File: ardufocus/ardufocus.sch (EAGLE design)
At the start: 14 parts, among them J5 POWER_JACK, M1 ARDUINO-NANO-3.0, X2 JST-XH-04-PIN-LONG-PAD, X3 JST-XH-04-PIN-LONG-PAD, X4 JST-XH-04-PIN-LONG-PAD, X5 JST-XH-04-PIN-LONG-PAD, X6 JST-XH-02-PIN-LONG-PAD

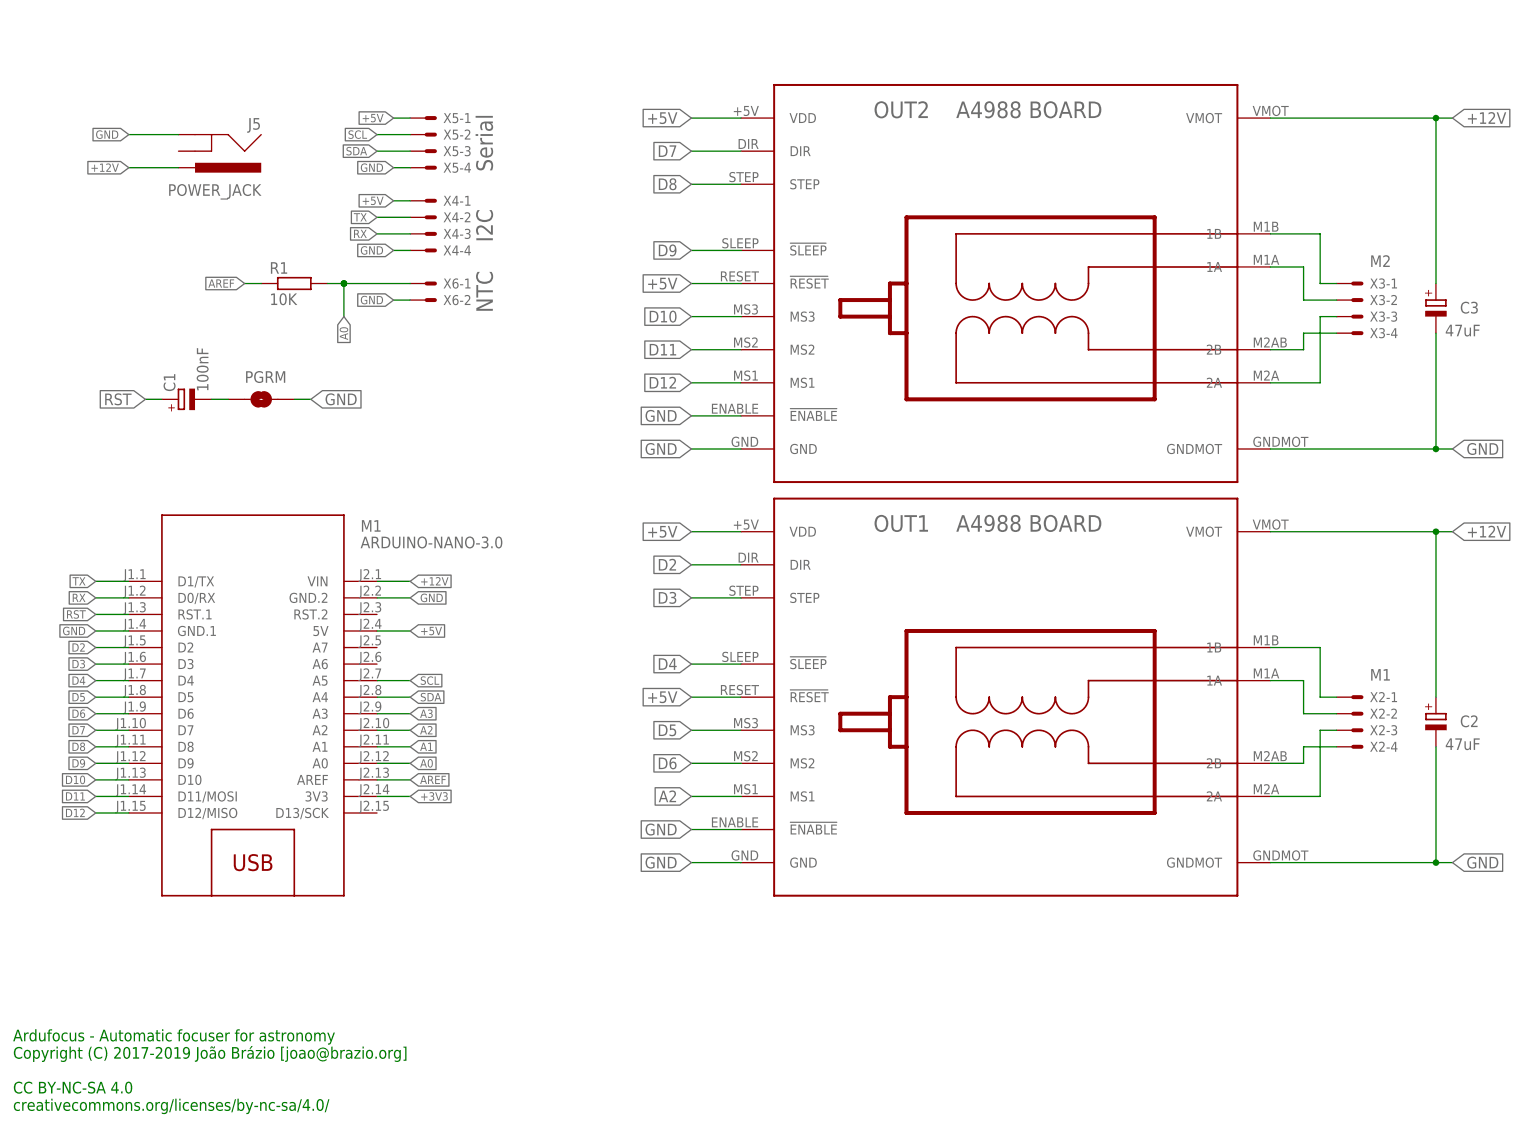
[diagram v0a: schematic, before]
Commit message: New PCB layout
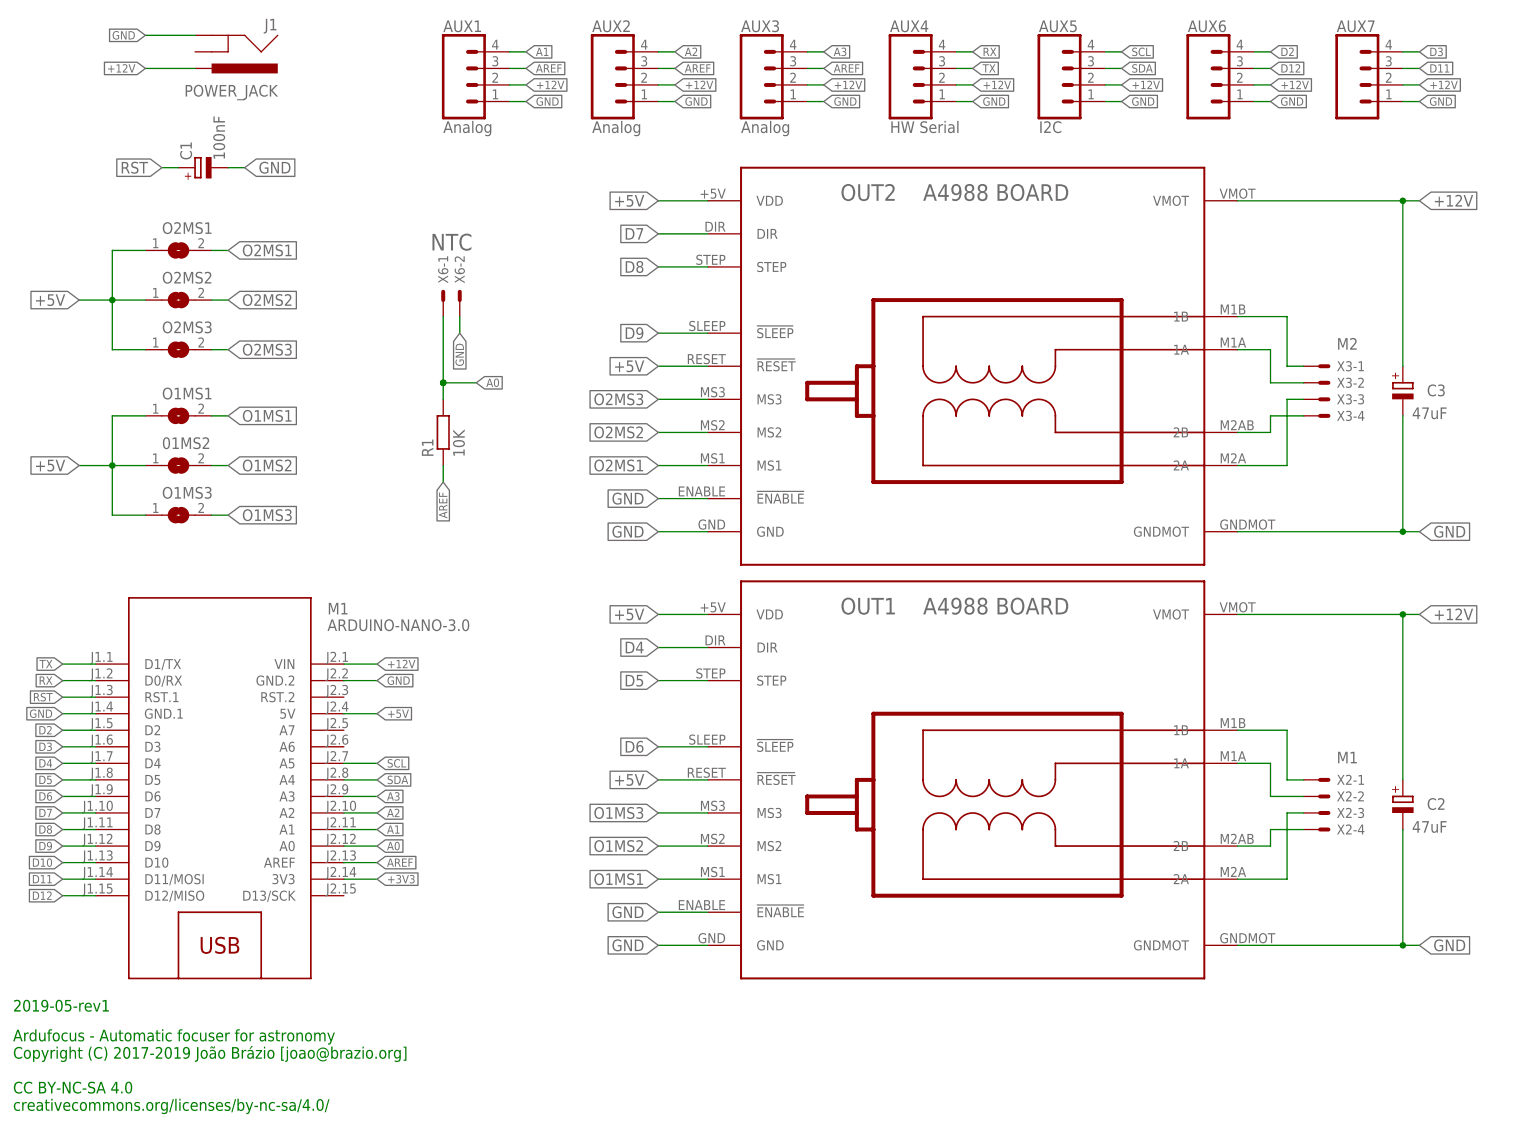
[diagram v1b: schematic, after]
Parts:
- removed J5: POWER_JACK, SparkFun-Connectors:POWER_JACK
- removed PGRM: JUMPER-SMT_2_NO_SILK, SparkFun-Jumpers:JUMPER-SMT_2_NO_SILK
- removed X4, X5: JST-XH-04-PIN-LONG-PAD, jst-xh:JST-XH-04-PIN-LONG-PAD
- added 01MS2, O1MS1, O1MS3, O2MS1, O2MS2, O2MS3: (no value), jumper:SJ
- added AUX1, AUX2, AUX3: Analog, SparkFun-Connectors:CONN_04
- added AUX4: HW Serial, SparkFun-Connectors:CONN_04
- added AUX5: I2C, SparkFun-Connectors:CONN_04
- added AUX6, AUX7: (no value), SparkFun-Connectors:CONN_04
- added J1: POWER_JACK, SparkFun-Connectors:POWER_JACK
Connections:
- removed net N$2: C1.-, PGRM.1
- new net O1MS1: O1MS1.2, OUT1.MS1
- new net O1MS2: 01MS2.2, OUT1.MS2
- new net O1MS3: O1MS3.2, OUT1.MS3
- new net O2MS1: O2MS1.2, OUT2.MS1
- new net O2MS2: O2MS2.2, OUT2.MS2
- new net O2MS3: O2MS3.2, OUT2.MS3
- net +12V: now also AUX1.2, AUX2.2, AUX3.2, AUX4.2, AUX5.2, AUX6.2, AUX7.2, J1.PWR; no longer J5.PWR
- net +5V: now also 01MS2.1, O1MS1.1, O1MS3.1, O2MS1.1, O2MS2.1, O2MS3.1; no longer X4-1.S, X5-1.S
- net A1: now also AUX1.4
- net A2: now also AUX2.4; no longer OUT1.MS1
- net A3: now also AUX3.4
- net AREF: now also AUX1.3, AUX2.3, AUX3.3
- net D10: no longer OUT2.MS3
- net D11: now also AUX7.3; no longer OUT2.MS2
- net D12: now also AUX6.3; no longer OUT2.MS1
- net D2: now also AUX6.4; no longer OUT1.DIR
- net D3: now also AUX7.4; no longer OUT1.STEP
- net D4: now also OUT1.DIR; no longer OUT1.!SLEEP
- net D5: now also OUT1.STEP; no longer OUT1.MS3
- net D6: now also OUT1.!SLEEP; no longer OUT1.MS2
- net GND: now also AUX1.1, AUX2.1, AUX3.1, AUX4.1, AUX5.1, AUX6.1, AUX7.1, C1.-, J1.GND; no longer J5.GND, PGRM.2, X4-4.S, X5-4.S
- net RX: now also AUX4.4; no longer X4-3.S
- net SCL: now also AUX5.4; no longer X5-2.S
- net SDA: now also AUX5.3; no longer X5-3.S
- net TX: now also AUX4.3; no longer X4-2.S
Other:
- note added: "2019-05-rev1"
- note removed: "I2C"
- note removed: "Serial"
- moved on the sheet: C1, C2, C3, M1, OUT1, OUT2, R1, X2-1, X2-2, X2-3, X2-4, X3-1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

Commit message: Revert "New PCB layout"
This reverts commit abb039d9954214917f7d505cd5213ebb6519a360.
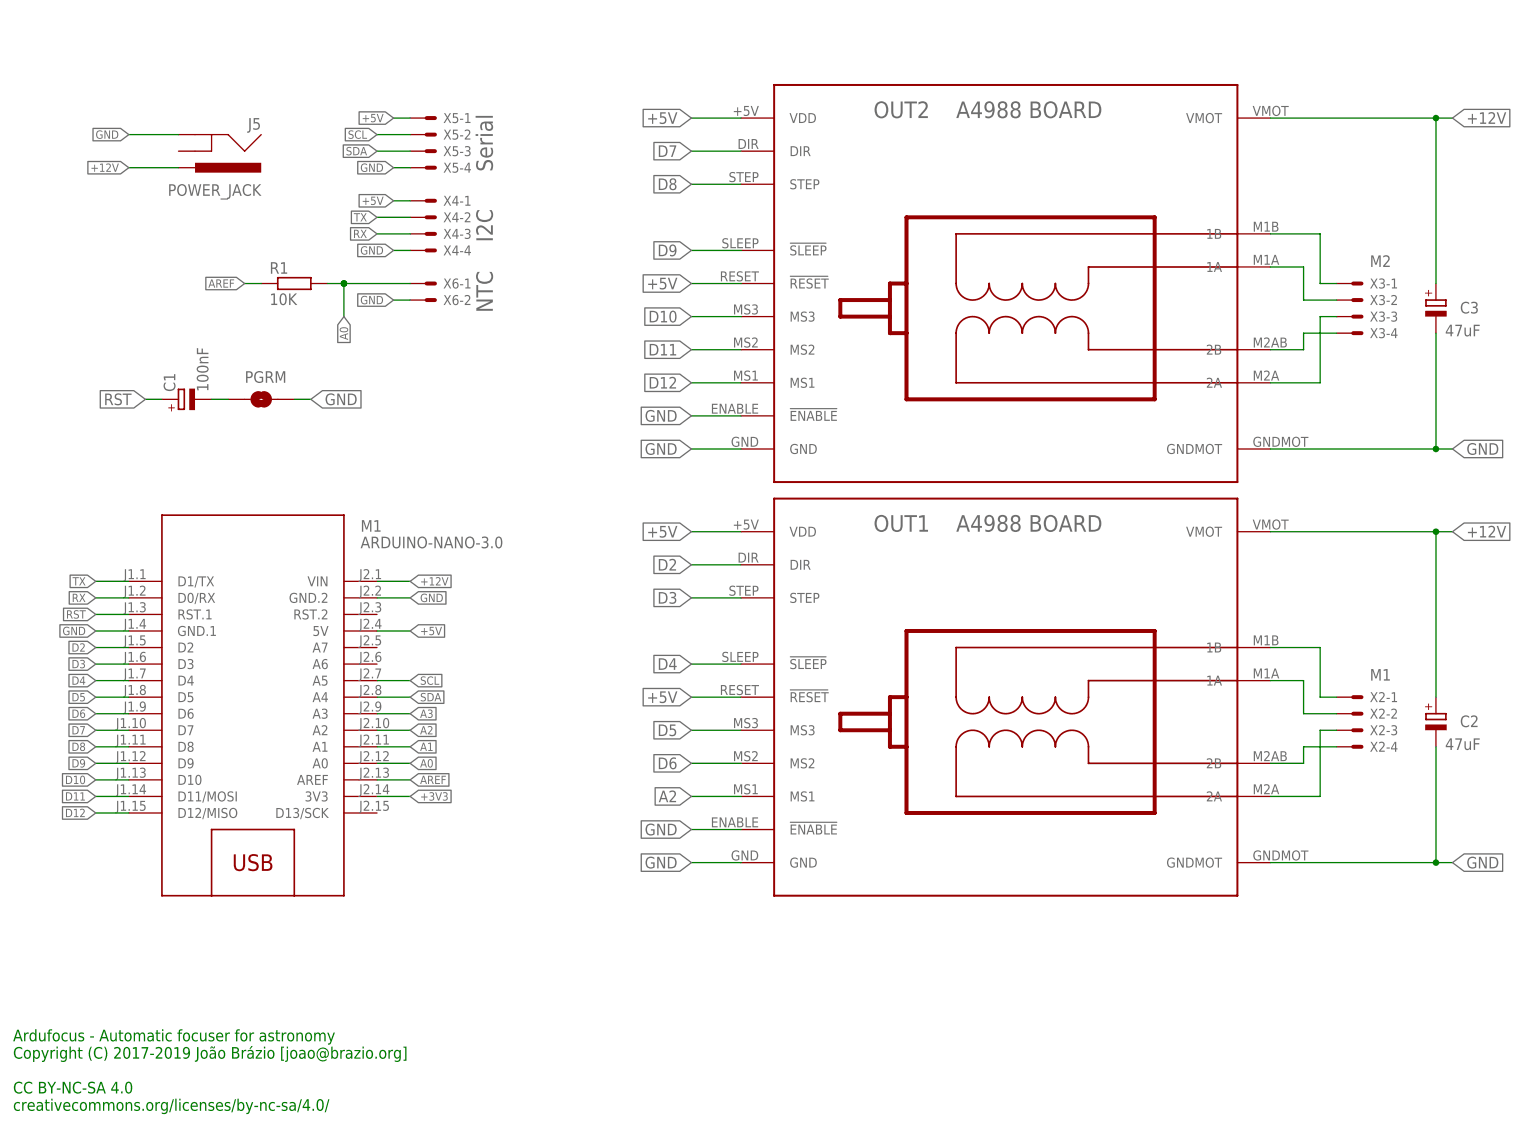
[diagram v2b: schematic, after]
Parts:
- removed 01MS2, O1MS1, O1MS3, O2MS1, O2MS2, O2MS3: (no value), jumper:SJ
- removed AUX1, AUX2, AUX3: Analog, SparkFun-Connectors:CONN_04
- removed AUX4: HW Serial, SparkFun-Connectors:CONN_04
- removed AUX5: I2C, SparkFun-Connectors:CONN_04
- removed AUX6, AUX7: (no value), SparkFun-Connectors:CONN_04
- removed J1: POWER_JACK, SparkFun-Connectors:POWER_JACK
- added J5: POWER_JACK, SparkFun-Connectors:POWER_JACK
- added PGRM: JUMPER-SMT_2_NO_SILK, SparkFun-Jumpers:JUMPER-SMT_2_NO_SILK
- added X4, X5: JST-XH-04-PIN-LONG-PAD, jst-xh:JST-XH-04-PIN-LONG-PAD
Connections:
- removed net O1MS1: O1MS1.2, OUT1.MS1
- removed net O1MS2: 01MS2.2, OUT1.MS2
- removed net O1MS3: O1MS3.2, OUT1.MS3
- removed net O2MS1: O2MS1.2, OUT2.MS1
- removed net O2MS2: O2MS2.2, OUT2.MS2
- removed net O2MS3: O2MS3.2, OUT2.MS3
- new net N$2: C1.-, PGRM.1
- net +12V: now also J5.PWR; no longer AUX1.2, AUX2.2, AUX3.2, AUX4.2, AUX5.2, AUX6.2, AUX7.2, J1.PWR
- net +5V: now also X4-1.S, X5-1.S; no longer 01MS2.1, O1MS1.1, O1MS3.1, O2MS1.1, O2MS2.1, O2MS3.1
- net A1: no longer AUX1.4
- net A2: now also OUT1.MS1; no longer AUX2.4
- net A3: no longer AUX3.4
- net AREF: no longer AUX1.3, AUX2.3, AUX3.3
- net D10: now also OUT2.MS3
- net D11: now also OUT2.MS2; no longer AUX7.3
- net D12: now also OUT2.MS1; no longer AUX6.3
- net D2: now also OUT1.DIR; no longer AUX6.4
- net D3: now also OUT1.STEP; no longer AUX7.4
- net D4: now also OUT1.!SLEEP; no longer OUT1.DIR
- net D5: now also OUT1.MS3; no longer OUT1.STEP
- net D6: now also OUT1.MS2; no longer OUT1.!SLEEP
- net GND: now also J5.GND, PGRM.2, X4-4.S, X5-4.S; no longer AUX1.1, AUX2.1, AUX3.1, AUX4.1, AUX5.1, AUX6.1, AUX7.1, C1.-, J1.GND
- net RX: now also X4-3.S; no longer AUX4.4
- net SCL: now also X5-2.S; no longer AUX5.4
- net SDA: now also X5-3.S; no longer AUX5.3
- net TX: now also X4-2.S; no longer AUX4.3
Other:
- note added: "I2C"
- note added: "Serial"
- note removed: "2019-05-rev1"
- moved on the sheet: C1, C2, C3, M1, OUT1, OUT2, R1, X2-1, X2-2, X2-3, X2-4, X3-1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
